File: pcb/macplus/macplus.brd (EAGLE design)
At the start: 54 x 32 mm, 10 parts, among them J1 ATX24RH

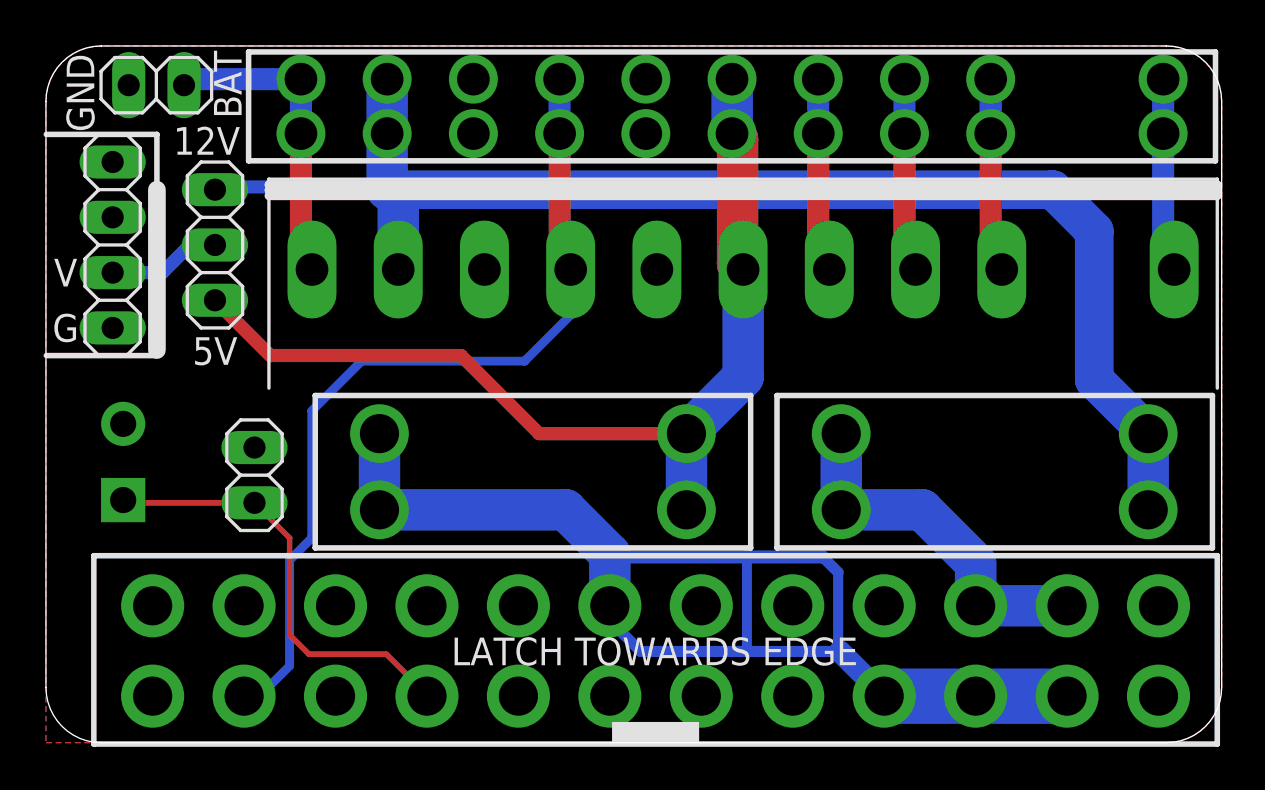
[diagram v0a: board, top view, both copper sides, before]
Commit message: updated mac SE pcb
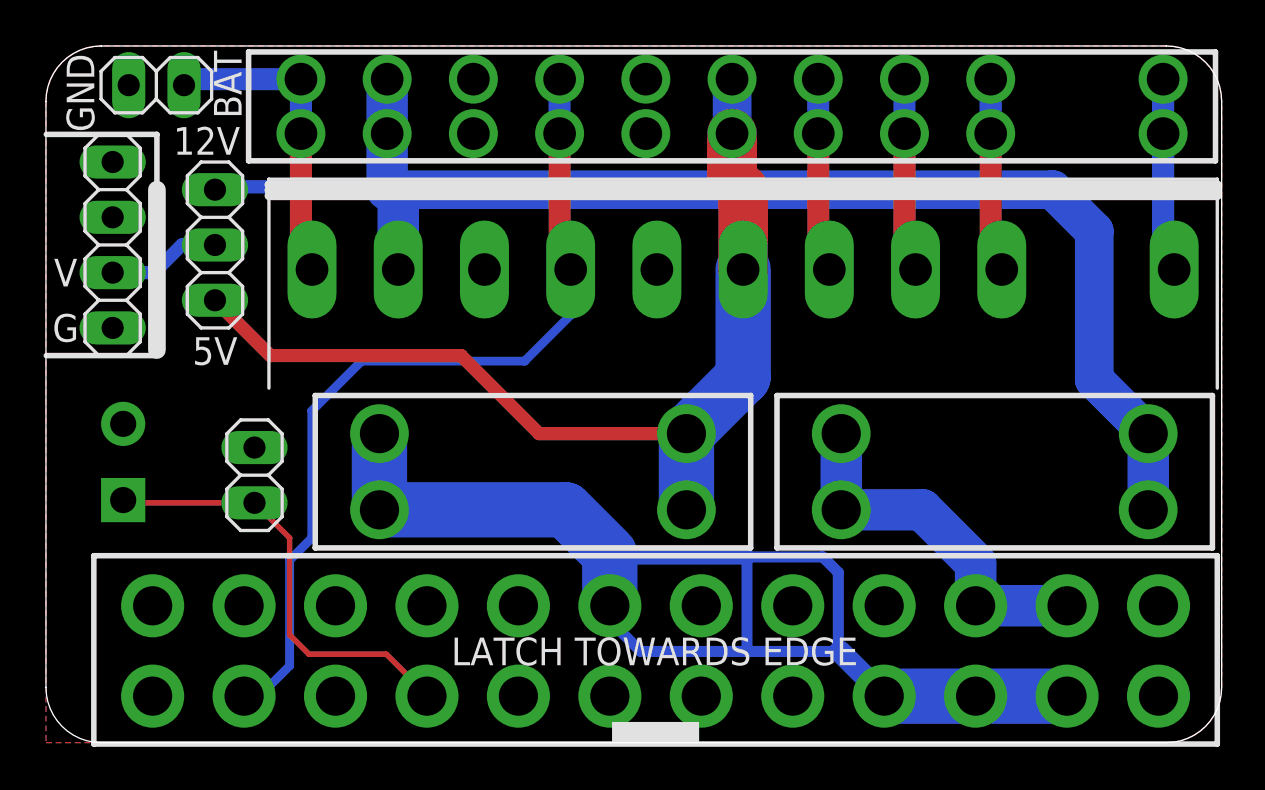
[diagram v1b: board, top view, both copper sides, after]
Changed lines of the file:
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@@
 <grid distance="5" unitdist="mil" unit="mil" style="lines" multiple="1" display="no" altdistance="1" altunitdist="mil" altunit="mil"/>
 <layers>
-<layer number="1" name="Top" color="4" fill="1" visible="no" active="yes"/>
+<layer number="1" name="Top" color="4" fill="1" visible="yes" active="yes"/>
 <layer number="2" name="Route2" color="16" fill="1" visible="no" active="no"/>
 <layer number="3" name="Route3" color="17" fill="1" visible="no" active="no"/>
@@
 <layer number="14" name="Route14" color="22" fill="1" visible="no" active="no"/>
 <layer number="15" name="Route15" color="23" fill="1" visible="no" active="no"/>
-<layer number="16" name="Bottom" color="1" fill="1" visible="no" active="yes"/>
+<layer number="16" name="Bottom" color="1" fill="1" visible="yes" active="yes"/>
 <layer number="17" name="Pads" color="2" fill="1" visible="yes" active="yes"/>
 <layer number="18" name="Vias" color="2" fill="1" visible="yes" active="yes"/>
@@
 <contactref element="U$3" pad="P$12"/>
 <contactref element="U$3" pad="P$11"/>
-<wire x1="30.418" y1="10.696" x2="30.418" y2="14.196" width="1.905" layer="16"/>
-<wire x1="30.418" y1="14.196" x2="33.02" y2="16.798" width="1.905" layer="16"/>
-<wire x1="33.02" y1="16.798" x2="33.02" y2="21.733" width="1.905" layer="16"/>
-<wire x1="32.512" y1="30.476" x2="32.512" y2="27.976" width="1.905" layer="16"/>
-<wire x1="32.512" y1="27.976" x2="32.766" y2="27.722" width="1.905" layer="1"/>
-<wire x1="32.766" y1="27.722" x2="32.766" y2="21.987" width="1.905" layer="1"/>
-<wire x1="32.766" y1="21.987" x2="33.02" y2="21.733" width="1.905" layer="1"/>
+<wire x1="30.418" y1="10.696" x2="30.418" y2="14.196" width="2.54" layer="16"/>
+<wire x1="30.418" y1="14.196" x2="33.02" y2="16.798" width="2.54" layer="16"/>
+<wire x1="33.02" y1="16.798" x2="33.02" y2="21.733" width="2.54" layer="16"/>
+<wire x1="32.512" y1="30.476" x2="32.512" y2="27.976" width="1.778" layer="16"/>
+<wire x1="33.02" y1="25.436" x2="32.512" y2="25.944" width="1.905" layer="1"/>
+<wire x1="32.512" y1="27.976" x2="32.512" y2="25.944" width="2.286" layer="1"/>
+<wire x1="33.02" y1="25.436" x2="33.02" y2="21.733" width="2.286" layer="1"/>
 <wire x1="30.418" y1="14.196" x2="23.65" y2="14.196" width="0.6096" layer="1"/>
 <wire x1="23.65" y1="14.196" x2="20.066" y2="17.78" width="0.6096" layer="1"/>
@@
 <wire x1="33.1978" y1="4.191" x2="37.465" y2="4.191" width="0.508" layer="16"/>
 <wire x1="39.5" y1="2.156" x2="39.5" y2="2.138" width="1.397" layer="16"/>
-<wire x1="26.9" y1="6.288" x2="26.9" y2="8.533" width="1.905" layer="16"/>
+<wire x1="26.9" y1="6.288" x2="26.9" y2="8.533" width="2.54" layer="16"/>
 <wire x1="26.9" y1="8.533" x2="26.9" y2="8.66" width="1.905" layer="16"/>
-<wire x1="24.864" y1="10.696" x2="16.318" y2="10.696" width="1.905" layer="16"/>
-<wire x1="26.9" y1="8.66" x2="24.864" y2="10.696" width="1.905" layer="16"/>
-<wire x1="16.318" y1="10.696" x2="16.318" y2="14.196" width="1.905" layer="16"/>
+<wire x1="24.864" y1="10.696" x2="16.318" y2="10.696" width="2.54" layer="16"/>
+<wire x1="26.9" y1="8.66" x2="24.864" y2="10.696" width="2.54" layer="16"/>
+<wire x1="16.318" y1="10.696" x2="16.318" y2="14.196" width="2.54" layer="16"/>
 <wire x1="28.321" y1="4.191" x2="26.9" y2="5.612" width="0.508" layer="16"/>
 <wire x1="26.9" y1="5.612" x2="26.9" y2="6.288" width="0.508" layer="16"/>
 <wire x1="39.5" y1="2.156" x2="37.465" y2="4.191" width="1.016" layer="16"/>
 <wire x1="37.465" y1="4.191" x2="37.3888" y2="4.2672" width="0.508" layer="16"/>
-<wire x1="37.3888" y1="4.2672" x2="37.3888" y2="7.8232" width="0.4572" layer="16"/>
+<wire x1="37.3888" y1="4.2672" x2="37.3888" y2="7.8232" width="0.508" layer="16"/>
 <wire x1="37.3888" y1="7.8232" x2="36.679" y2="8.533" width="0.508" layer="16"/>
-<wire x1="36.679" y1="8.533" x2="33.1978" y2="8.533" width="0.6096" layer="16"/>
-<wire x1="33.1978" y1="8.533" x2="26.9" y2="8.533" width="0.6096" layer="16"/>
-<wire x1="33.1978" y1="8.533" x2="33.1978" y2="4.191" width="0.4572" layer="16"/>
+<wire x1="36.679" y1="8.533" x2="33.1978" y2="8.533" width="0.508" layer="16"/>
+<wire x1="33.1978" y1="8.533" x2="26.9" y2="8.533" width="0.7112" layer="16"/>
+<wire x1="33.1978" y1="8.533" x2="33.1978" y2="4.191" width="0.508" layer="16"/>
 </signal>
 <signal name="N$8">
@@
 <contactref element="JP4" pad="3"/>
 <contactref element="JP1" pad="2"/>
-<wire x1="8.763" y1="22.86" x2="7.62" y2="22.86" width="0.6096" layer="16"/>
-<wire x1="6.35" y1="21.59" x2="4.064" y2="21.59" width="0.6096" layer="16"/>
-<wire x1="7.62" y1="22.86" x2="6.35" y2="21.59" width="0.6096" layer="16"/>
+<wire x1="8.763" y1="22.86" x2="7.239" y2="22.86" width="0.6096" layer="16"/>
+<wire x1="5.969" y1="21.59" x2="4.064" y2="21.59" width="0.6096" layer="16"/>
+<wire x1="7.239" y1="22.86" x2="5.969" y2="21.59" width="0.6096" layer="16"/>
 </signal>
 </signals>
